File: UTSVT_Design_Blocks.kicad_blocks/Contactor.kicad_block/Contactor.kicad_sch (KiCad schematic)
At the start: 15 parts

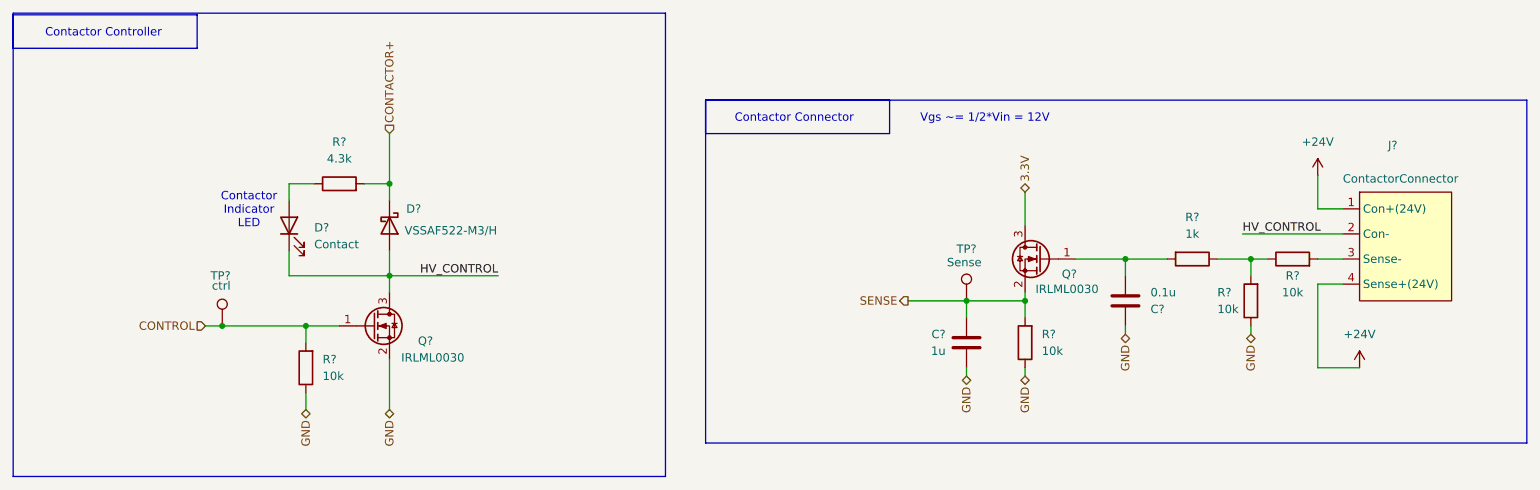
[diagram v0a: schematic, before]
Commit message: fixed footprints + 3d models
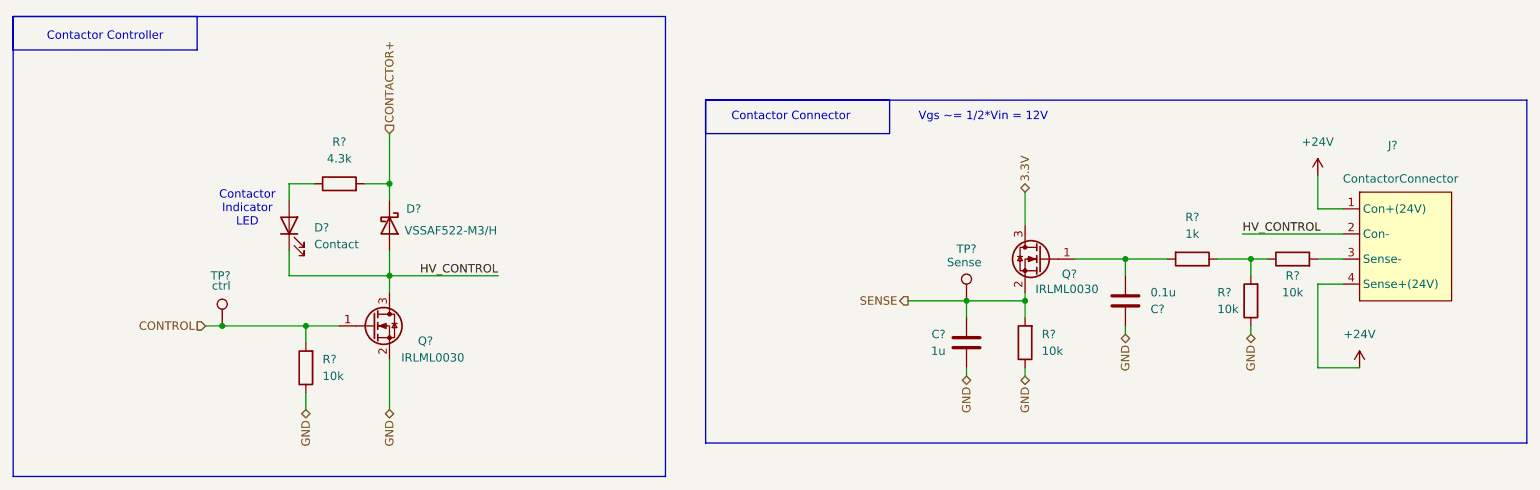
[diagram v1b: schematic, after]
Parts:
- D?: footprint CustomKiCad-Library:SODFL5226X100N -> LHRS_Passives:SODFL5226X100N
- J?: footprint UTSVT_Connectors:Molex_Nano-Fit_105309-xx04_1x04_P2.50mm_Vertical -> LHRS_Connectors:Molex_Nano-Fit_105309-xx05_1x04_P2.50mm_Vertical
- R? (x6): footprint (none) -> Resistor_SMD:R_0603_1608Metric_Pad0.98x0.95mm_HandSolder
- TP? (x2): footprint TestPoint:TestPoint_Pad_1.0x1.0mm -> TestPoint:TestPoint_THTPad_D3.0mm_Drill1.5mm
